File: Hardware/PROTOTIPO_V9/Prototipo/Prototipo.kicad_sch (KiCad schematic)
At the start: 1 part, among them U1 YAAJ_BluePill_Part_Like_SWD_B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

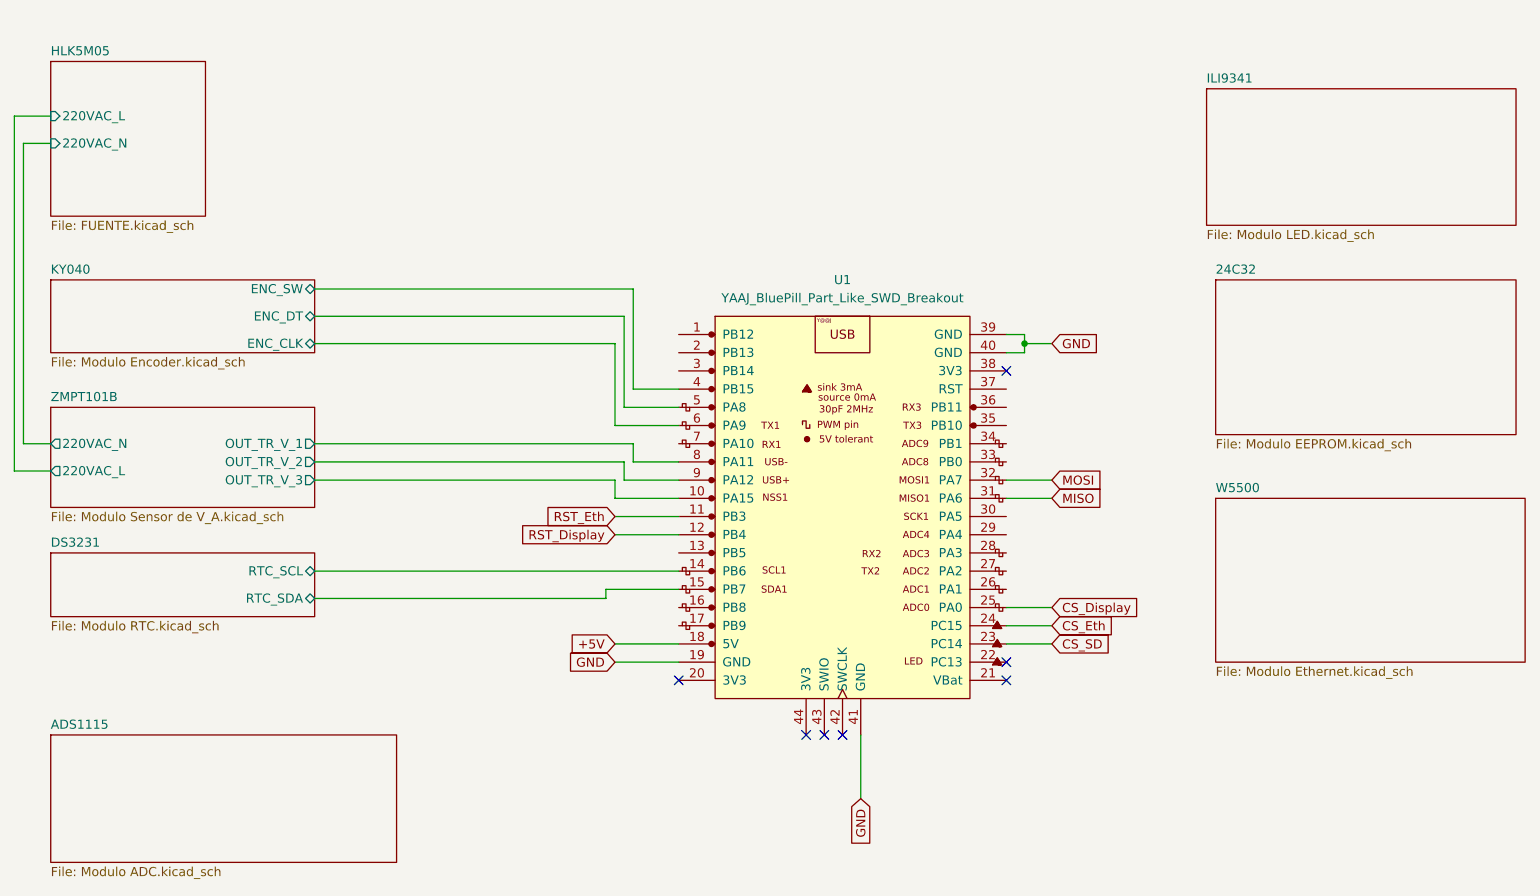
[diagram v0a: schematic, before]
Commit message: Bus de salida
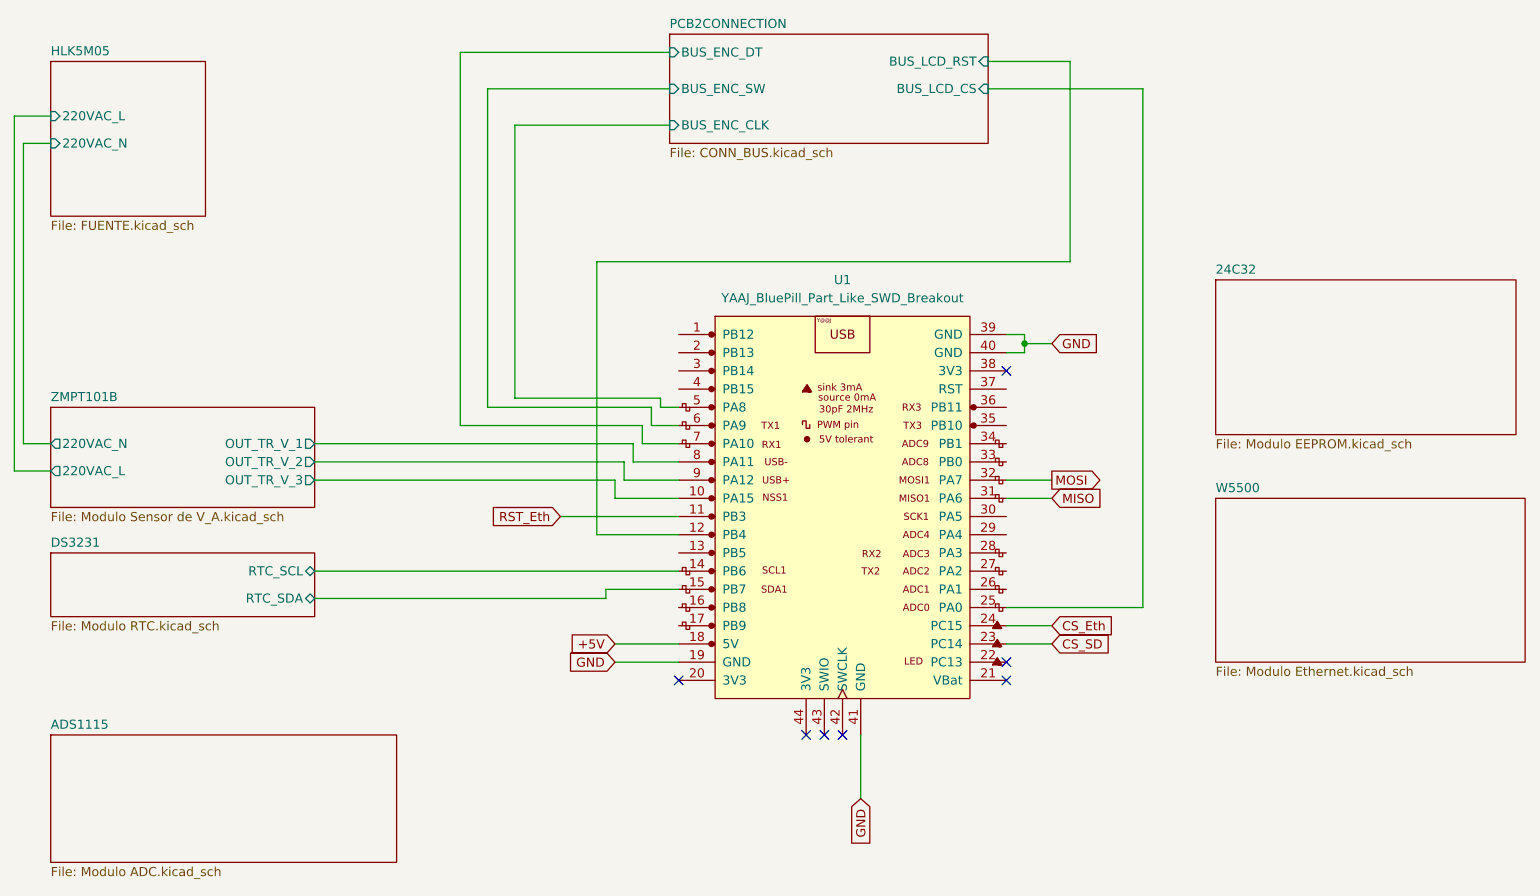
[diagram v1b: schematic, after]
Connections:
- net PCB2CONNECTION/BUS_ENC_DT: now reaches U1.7 (PA10)
- net CS_Display renamed PCB2CONNECTION/BUS_LCD_CS
- net KY040/ENC_CLK renamed PCB2CONNECTION/BUS_ENC_SW
- net KY040/ENC_DT renamed PCB2CONNECTION/BUS_ENC_CLK
- net KY040/ENC_SW: no longer names the net of U1.4 (PB15)
- net RST_Display renamed PCB2CONNECTION/BUS_LCD_RST
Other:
- removed sheet ILI9341
- removed sheet KY040
- added sheet PCB2CONNECTION (CONN_BUS.kicad_sch)
